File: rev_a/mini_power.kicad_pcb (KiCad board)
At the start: 2 copper layers, 4 parts

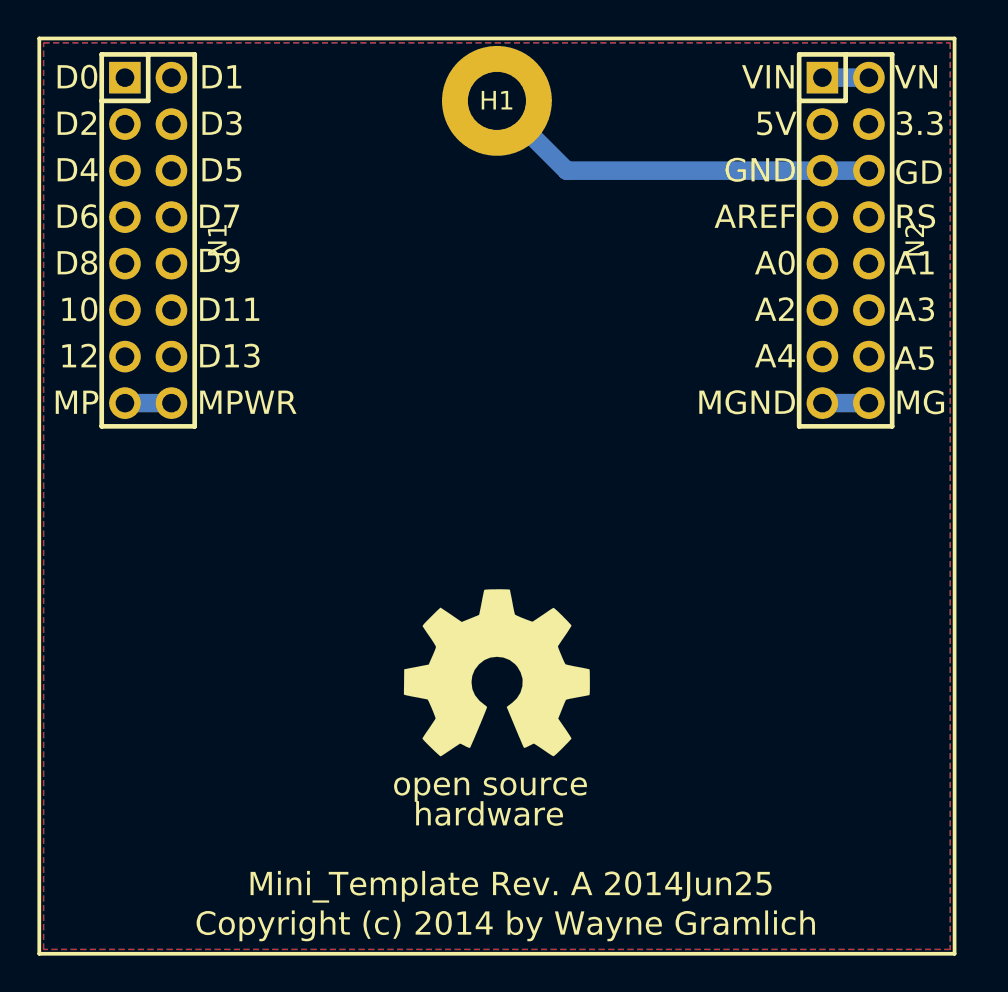
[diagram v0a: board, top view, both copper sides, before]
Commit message: Did initial board layout.
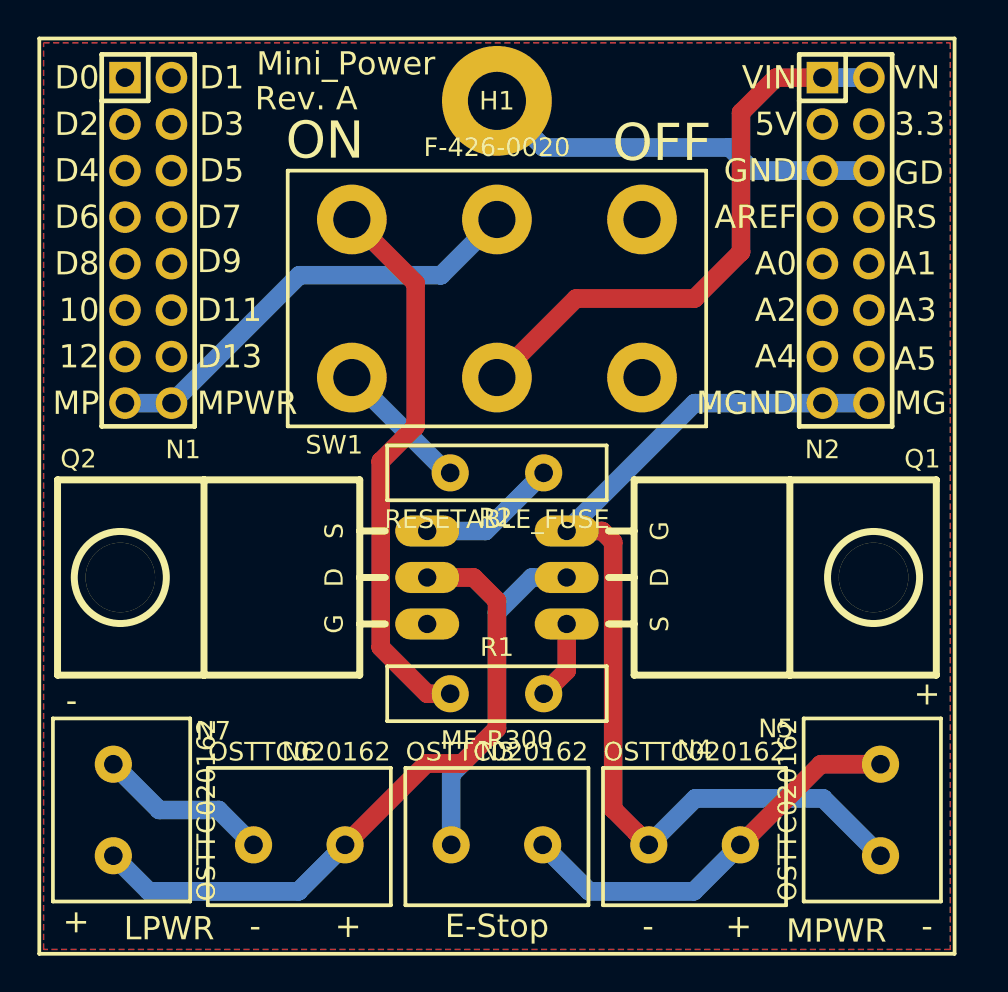
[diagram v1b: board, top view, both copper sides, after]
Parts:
- added N3: OSTTC020162, Mini_Power_Rev_A:5MM_TERMINAL_BLOCK_2_POS, F.Cu at (101.6, 147.3)
- added N4: OSTTC020162, Mini_Power_Rev_A:5MM_TERMINAL_BLOCK_2_POS, F.Cu at (112.4, 147.3)
- added N5: OSTTC020162, Mini_Power_Rev_A:5MM_TERMINAL_BLOCK_2_POS, F.Cu at (122.6, 145.4)
- added N6: OSTTC020162, Mini_Power_Rev_A:5MM_TERMINAL_BLOCK_2_POS, F.Cu at (90.8, 147.3)
- added N7: OSTTC020162, Mini_Power_Rev_A:5MM_TERMINAL_BLOCK_2_POS, F.Cu at (80.6, 145.4)
- added Q1: FQP47P06, Mini_Power_Rev_A:TO-220_FET-GDS_Horizontal_LargePads, F.Cu at (105.4, 132.7)
- added Q2: FQP47P06, Mini_Power_Rev_A:TO-220_FET-GDS_Horizontal_LargePads, F.Cu at (97.8, 132.7)
- added R1: MF-R300, Mini_Power_Rev_A:MF_R300, F.Cu at (101.6, 139.1)
- added R2: RESETABLE_FUSE, Mini_Power_Rev_A:MF_R300, F.Cu at (101.6, 127.0)
- added SW1: F-426-0020, Mini_Power_Rev_A:GF_426_0020, F.Cu at (101.6, 117.5)
- G1: moved to B.Cu
- N1: value MS_DATA_HEADER -> MS_DATA_HEADER_POWER
- N2: value MS_PWR_HEADER -> MS_PWR_HEADER_POWER
- moved G1 13.1 mm to (89.5, 132.7)
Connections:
- N1 pad 1: /D0 -> (no net)
- N1 pad 10: /D9 -> (no net)
- N1 pad 11: /D10 -> (no net)
- N1 pad 12: /D11 -> (no net)
- N1 pad 13: /D12 -> (no net)
- N1 pad 14: /D13 -> (no net)
- N1 pad 2: /D1 -> (no net)
- N1 pad 3: /D2 -> (no net)
- N1 pad 4: /D3 -> (no net)
- N1 pad 5: /D4 -> (no net)
- N1 pad 6: /D5 -> (no net)
- N1 pad 7: /D6 -> (no net)
- N1 pad 8: /D7 -> (no net)
- N1 pad 9: /D8 -> (no net)
- N2 pad 10: /A1 -> (no net)
- N2 pad 11: /A2 -> (no net)
- N2 pad 12: /A3 -> (no net)
- N2 pad 13: /A4 -> (no net)
- N2 pad 14: /A5 -> (no net)
- N2 pad 3: /5V -> (no net)
- N2 pad 4: /3V3 -> (no net)
- N2 pad 7: /AREF -> (no net)
- N2 pad 8: /~RESET -> (no net)
- N2 pad 9: /A0 -> (no net)
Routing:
- net /MGND: track 2.54 -> 55.5 mm
- net /LPWR1: track 0.00 -> 36.8 mm
- net /MPWR3: track 0.00 -> 30.4 mm
- net /VIN: track 2.54 -> 31.6 mm
- net /LPWR4: track 0.00 -> 22.4 mm
- net /MPWR: track 2.54 -> 24.5 mm
- net /MPWR1: track 0.00 -> 18.3 mm
- net /GND: track 21.9 -> 31.4 mm
- net /LPWR2: track 0.00 -> 7.68 mm
- net /LPWR3: track 0.00 -> 7.53 mm
- net /MPWR2: track 0.00 -> 4.33 mm
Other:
- board text added: "+"
- board text added: "-"
- board text added: "E-Stop"
- board text added: "LPWR"
- board text added: "Mini_Power"
- board text added: "OFF"
- board text added: "ON"
- board text added: "Power Mini-Shield Rev. A Copyright (c) 2014 - Gramlich"
- board text added: "Rev. A"
- board text removed: "Copyright (c) 2014 by Wayne Gramlich"
- board text removed: "Mini_Template Rev. A 2014Jun25"
